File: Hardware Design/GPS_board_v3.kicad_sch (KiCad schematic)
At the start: 15 parts, among them IC2 SN65HVD231QDR, U1 STM32F042F4Px, U5 MAX-M8W

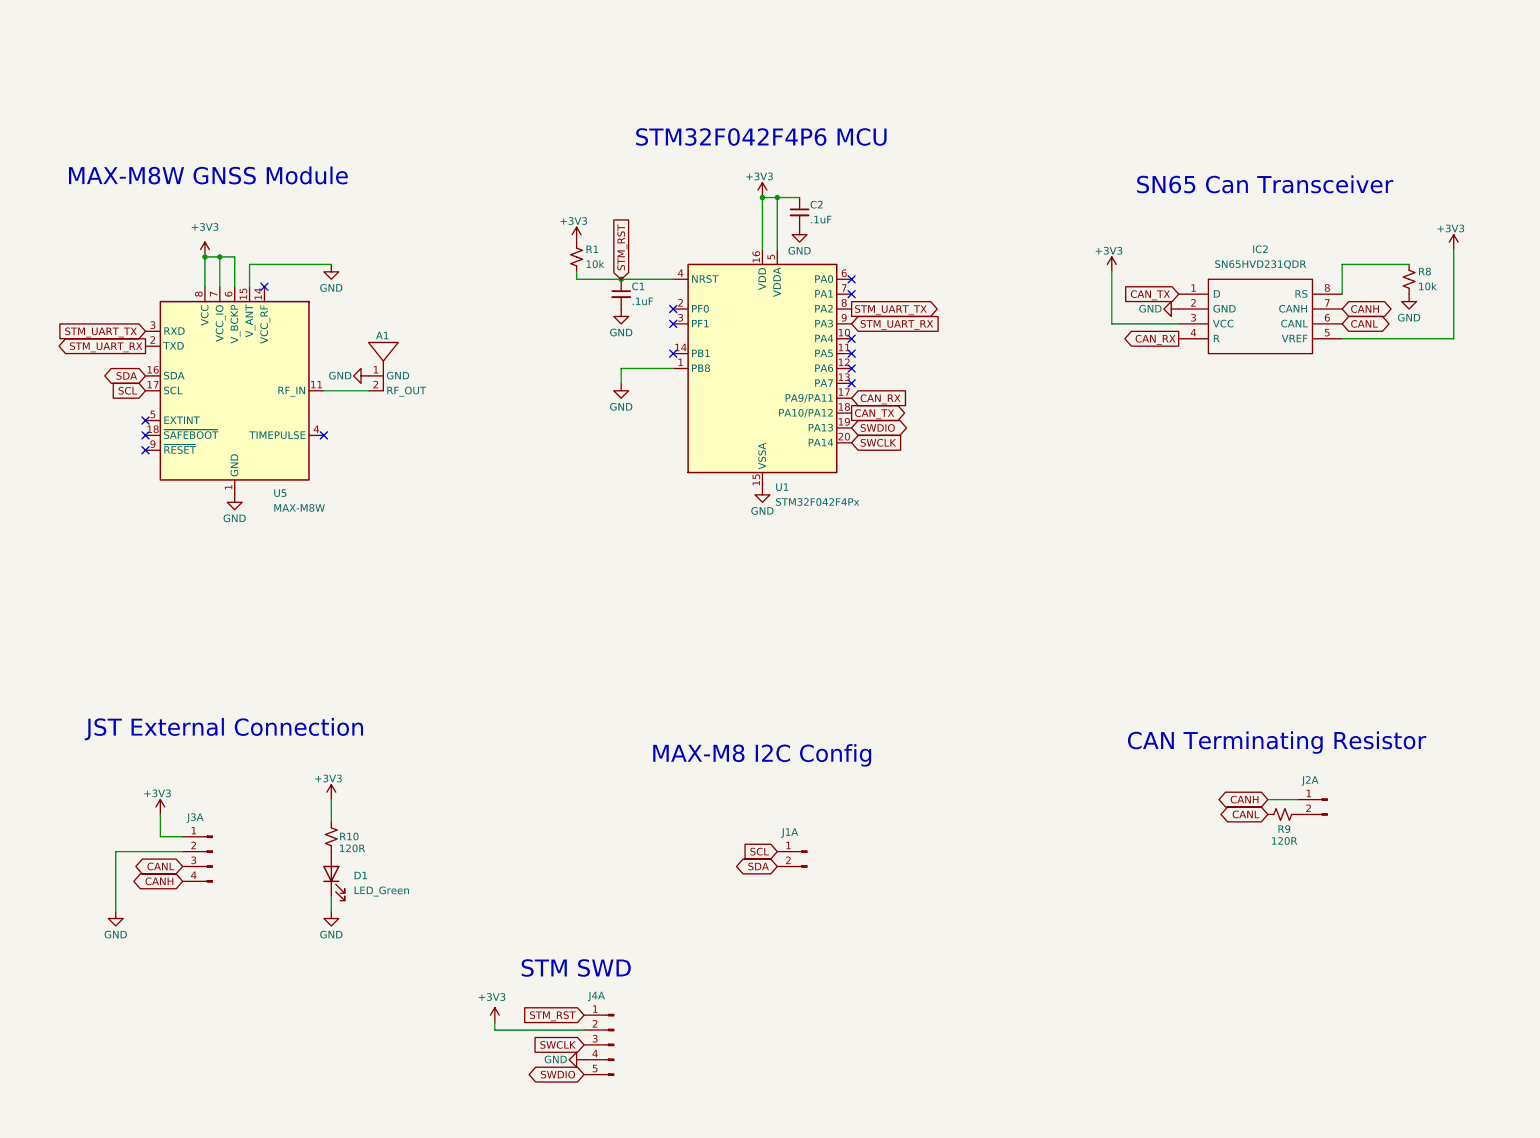
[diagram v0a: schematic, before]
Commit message: final updated board + prod files
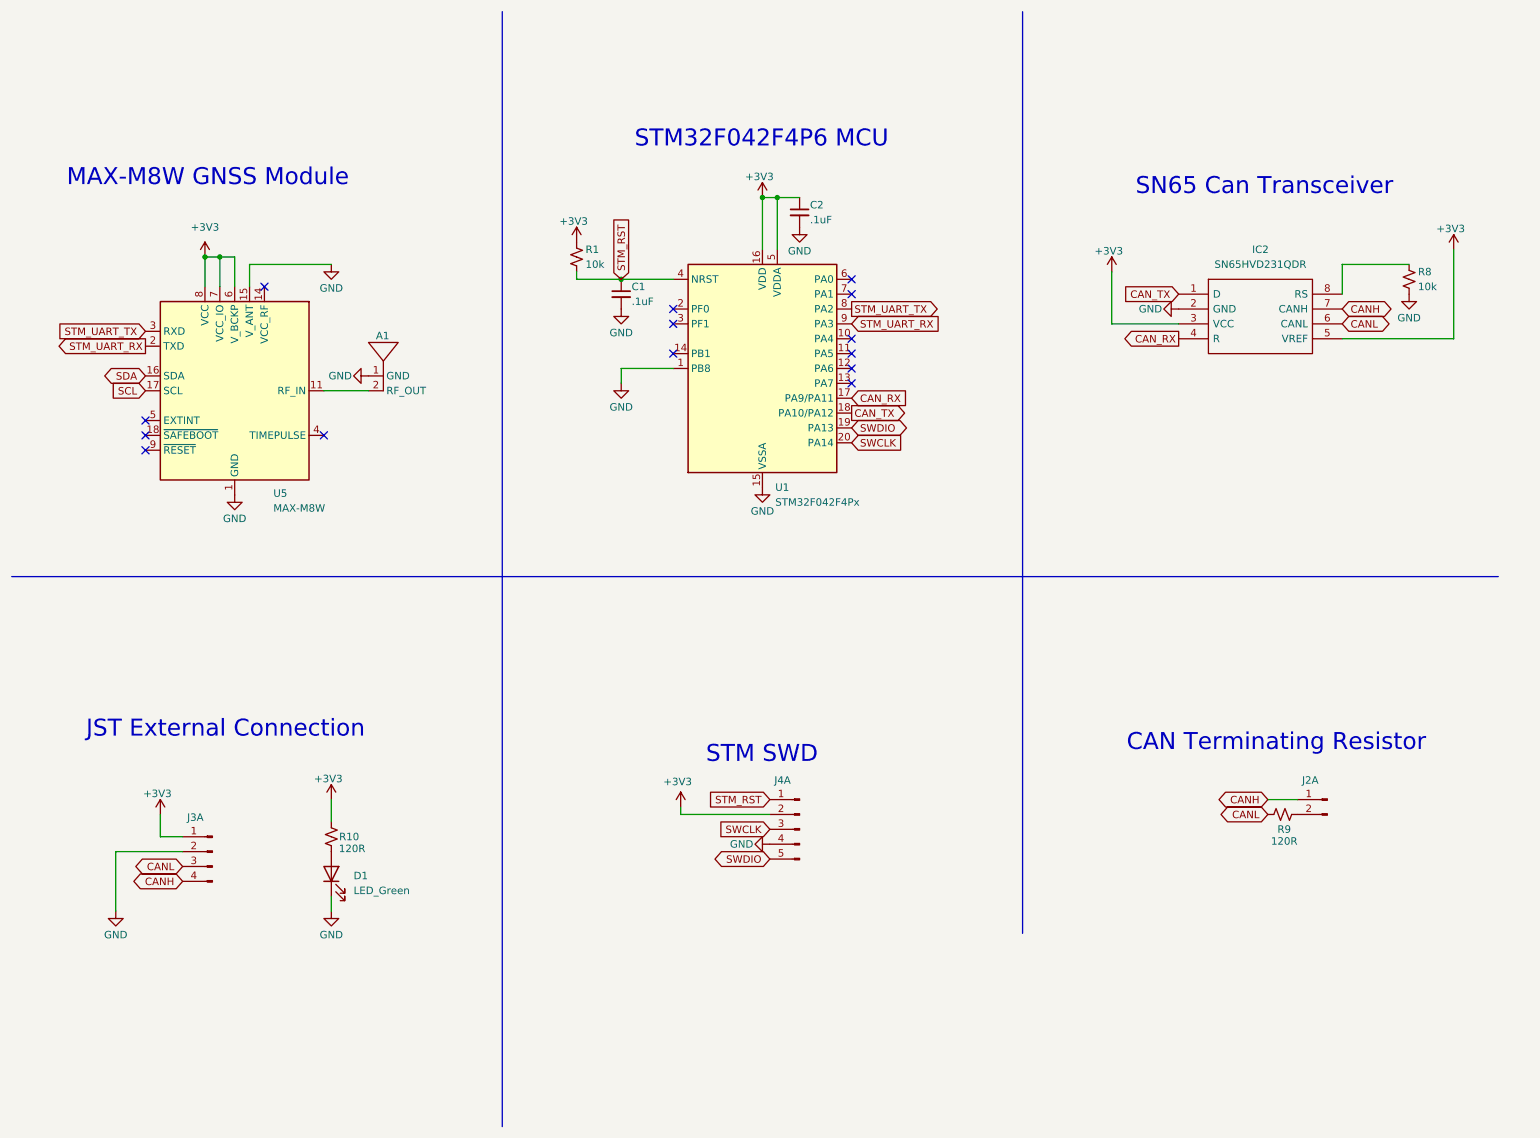
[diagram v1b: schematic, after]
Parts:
- removed J1: ~, Connector_PinHeader_2.54mm:PinHeader_1x02_P2.54mm_Vertical, symbol Connector:Samtec_ASP-134486-01
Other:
- note removed: "MAX-M8 I2C Config"
- moved on the sheet: J4A
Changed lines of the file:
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@@
 	(wire
 		(pts
-			(xy 95.25 185.42) (xy 95.25 186.69)
+			(xy 127 148.59) (xy 127 149.86)
 		)
 		(stroke
@@
 		)
 	)
+	(polyline
+		(pts
+			(xy 12.7 109.22) (xy 96.52 109.22)
+		)
+		(stroke
+			(width 0)
+			(type default)
+		)
+	)
+	(polyline
+		(pts
+			(xy 185.42 12.7) (xy 185.42 170.18)
+		)
+		(stroke
+			(width 0)
+			(type default)
+		)
+	)
 	(wire
 		(pts
-			(xy 95.25 186.69) (xy 110.49 186.69)
+			(xy 127 149.86) (xy 142.24 149.86)
 		)
 		(stroke
@@
 		)
 	)
+	(polyline
+		(pts
+			(xy 96.52 12.7) (xy 96.52 203.2)
+		)
+		(stroke
+			(width 0)
+			(type default)
+		)
+	)
 	(wire
 		(pts
@@
 		)
 	)
+	(polyline
+		(pts
+			(xy 96.52 109.22) (xy 266.7 109.22)
+		)
+		(stroke
+			(width 0)
+			(type default)
+		)
+	)
 	(text "MAX-M8W GNSS Module"
 		(exclude_from_sim no)
@@
 		)
 	)
-	(text "MAX-M8 I2C Config"
-		(exclude_from_sim no)
-		(at 121.92 138.0744 0)
-		(effects
-			(font
-				(face "KiCad Font")
-				(size 2.8956 2.8956)
-			)
-			(justify left top)
-		)
-	)
 	(text "STM SWD"
 		(exclude_from_sim no)
-		(at 99.568 174.752 0)
+		(at 131.318 137.922 0)
 		(effects
 			(font
@@
 	(global_label "SWCLK"
 		(shape input)
-		(at 110.49 189.23 180)
+		(at 142.24 152.4 180)
 		(fields_autoplaced yes)
 		(effects
@@
 		)
 		(property "Intersheetrefs" "${INTERSHEET_REFS}"
-			(at 101.2758 189.23 0)
+			(at 133.0258 152.4 0)
 			(effects
 				(font
@@
 		)
 	)
-	(global_label "SCL"
-		(shape input)
-		(at 143.51 156.21 180)
-		(effects
-			(font
-				(size 1.27 1.27)
-			)
-			(justify right)
-		)
-		(property "Intersheetrefs" "${INTERSHEET_REFS}"
-			(at 143.51 156.21 0)
-			(effects
-				(font
-					(size 1.27 1.27)
-				)
-				(hide yes)
-			)
-		)
-	)
 	(global_label "CAN_RX"
 		(shape output)
@@
 		)
 	)
-	(global_label "SDA"
-		(shape bidirectional)
-		(at 143.51 158.75 180)
-		(effects
-			(font
-				(size 1.27 1.27)
-			)
-			(justify right)
-		)
-		(property "Intersheetrefs" "${INTERSHEET_REFS}"
-			(at 143.51 158.75 0)
-			(effects
-				(font
-					(size 1.27 1.27)
-				)
-				(hide yes)
-			)
-		)
-	)
 	(global_label "SCL"
 		(shape input)
@@
 	(global_label "STM_RST"
 		(shape input)
-		(at 110.49 184.15 180)
+		(at 142.24 147.32 180)
 		(fields_autoplaced yes)
 		(effects
@@
 		)
 		(property "Intersheetrefs" "${INTERSHEET_REFS}"
-			(at 99.4616 184.15 0)
+			(at 131.2116 147.32 0)
 			(effects
 				(font
@@
 	(global_label "SWDIO"
 		(shape bidirectional)
-		(at 110.49 194.31 180)
+		(at 142.24 157.48 180)
 		(fields_autoplaced yes)
 		(effects
@@
 		)
 		(property "Intersheetrefs" "${INTERSHEET_REFS}"
-			(at 100.5273 194.31 0)
+			(at 132.2773 157.48 0)
 			(effects
 				(font
@@
 	(symbol
 		(lib_id "power:GND")
-		(at 110.49 191.77 270)
+		(at 142.24 154.94 270)
 		(unit 1)
 		(exclude_from_sim no)
@@
 		(dnp no)
 		(property "Reference" "#PWR018"
-			(at 104.14 191.77 0)
+			(at 135.89 154.94 0)
 			(effects
 				(font
@@
 		)
 		(property "Value" "GND"
-			(at 105.664 191.77 90)
+			(at 137.414 154.94 90)
 			(effects
 				(font
@@
 		)
 		(property "Footprint" ""
-			(at 110.49 191.77 0)
+			(at 142.24 154.94 0)
 			(effects
 				(font
@@
 		)
 		(property "Datasheet" ""
-			(at 110.49 191.77 0)
+			(at 142.24 154.94 0)
 			(effects
 				(font
@@
 		)
 		(property "Description" "Power symbol creates a global label with name \"GND\" , ground"
-			(at 110.49 191.77 0)
+			(at 142.24 154.94 0)
 			(effects
 				(font
@@
 	(symbol
 		(lib_id "power:+3V3")
-		(at 95.25 185.42 0)
+		(at 127 148.59 0)
 		(unit 1)
 		(exclude_from_sim no)
@@
 		(dnp no)
 		(property "Reference" "#PWR019"
-			(at 95.25 189.23 0)
+			(at 127 152.4 0)
 			(effects
 				(font
@@
 		)
 		(property "Value" "+3V3"
-			(at 94.742 181.102 0)
+			(at 126.492 144.272 0)
 			(effects
 				(font
@@
 		)
 		(property "Footprint" ""
-			(at 95.25 185.42 0)
+			(at 127 148.59 0)
 			(effects
 				(font
@@
 		)
 		(property "Datasheet" ""
-			(at 95.25 185.42 0)
+			(at 127 148.59 0)
 			(effects
 				(font
@@
 		)
 		(property "Description" "Power symbol creates a global label with name \"+3V3\""
-			(at 95.25 185.42 0)
+			(at 127 148.59 0)
 			(effects
 				(font
@@
 		(lib_name "Samtec_ASP-134486-01_2")
 		(lib_id "Connector:Samtec_ASP-134486-01")
-		(at 113.03 177.8 0)
+		(at 144.78 140.97 0)
 		(unit 1)
 		(exclude_from_sim no)
@@
 		(fields_autoplaced yes)
 		(property "Reference" "J4"
-			(at 111.252 180.848 0)
+			(at 143.002 144.018 0)
 			(effects
 				(font
@@
 		)
 		(property "Value" "~"
-			(at 100.838 180.848 0)
+			(at 132.588 144.018 0)
 			(effects
 				(font
@@
 		)
 		(property "Footprint" "Connector_PinHeader_2.54mm:PinHeader_1x05_P2.54mm_Vertical"
-			(at 114.3 123.19 0)
+			(at 146.05 86.36 0)
 			(effects
 				(font
@@
 		)
 		(property "Datasheet" "http://suddendocs.samtec.com/prints/asp-134486-01-mkt.pdf"
-			(at 116.84 124.46 0)
+			(at 148.59 87.63 0)
 			(effects
 				(font
@@
 		)
 		(property "Description" "Connector array, 10x40, 1.27mm pitch, carrier-card, receptacle, gold finish, VITA 57.1 FMC, SMD"
-			(at 113.03 177.8 0)
+			(at 144.78 140.97 0)
 			(effects
 				(font
@@
 					(unit 1)
 				)
-			)
-		)
-	)
-	(symbol
-		(lib_id "Connector:Samtec_ASP-134486-01")
-		(at 146.05 149.86 0)
-		(unit 1)
-		(exclude_from_sim no)
-		(in_bom yes)
-		(on_board yes)
-		(dnp no)
-		(fields_autoplaced yes)
-		(property "Reference" "J1"
-			(at 144.272 152.908 0)
-			(effects
-				(font
-					(size 1.27 1.27)
-				)
-				(justify left)
-			)
-		)
-		(property "Value" "~"
-			(at 133.858 152.908 0)
-			(effects
-				(font
-					(size 1.27 1.27)
-				)
-				(justify left)
-			)
-		)
-		(property "Footprint" "Connector_PinHeader_2.54mm:PinHeader_1x02_P2.54mm_Vertical"
-			(at 147.32 95.25 0)
-			(effects
-				(font
-					(size 1.27 1.27)
-				)
-				(hide yes)
-			)
-		)
-		(property "Datasheet" "http://suddendocs.samtec.com/prints/asp-134486-01-mkt.pdf"
-			(at 149.86 96.52 0)
-			(effects
-				(font
-					(size 1.27 1.27)
-				)
-				(hide yes)
-			)
-		)
-		(property "Description" "Connector array, 10x40, 1.27mm pitch, carrier-card, receptacle, gold finish, VITA 57.1 FMC, SMD"
-			(at 146.05 149.86 0)
-			(effects
-				(font
-					(size 1.27 1.27)
-				)
-				(hide yes)
-			)
-		)
-		(pin "H2"
-		)
-		(pin "J1"
-		)
-		(pin "J2"
-		)
-		(pin "K1"
-		)
-		(pin "K2"
-		)
-		(pin "C1"
-		)
-		(pin "E2"
-		)
-		(pin "G2"
-		)
-		(pin "E1"
-		)
-		(pin "F2"
-		)
-		(pin "D1"
-		)
-		(pin "B1"
-		)
-		(pin "B2"
-		)
-		(pin "D2"
-		)
-		(pin "1"
-		)
-		(pin "F1"
-		)
-		(pin "H1"
-		)
-		(pin "2"
-		)
-		(pin "C2"
-		)
-		(pin "G1"
-		)
-		(instances
-			(project "GPS_board_v3"
-				(path "/c3e0ad51-8a79-42ff-b905-b5467e5e45fa"
-					(reference "J1")
-					(unit 1)
-				)
